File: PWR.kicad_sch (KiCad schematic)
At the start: 32 parts, among them J1 Conn_01x02_Pin, U2 XC6206P332MR, U4 MCP6001-OT, U5 AMS1117-3.3, U6 XL1509-5.0

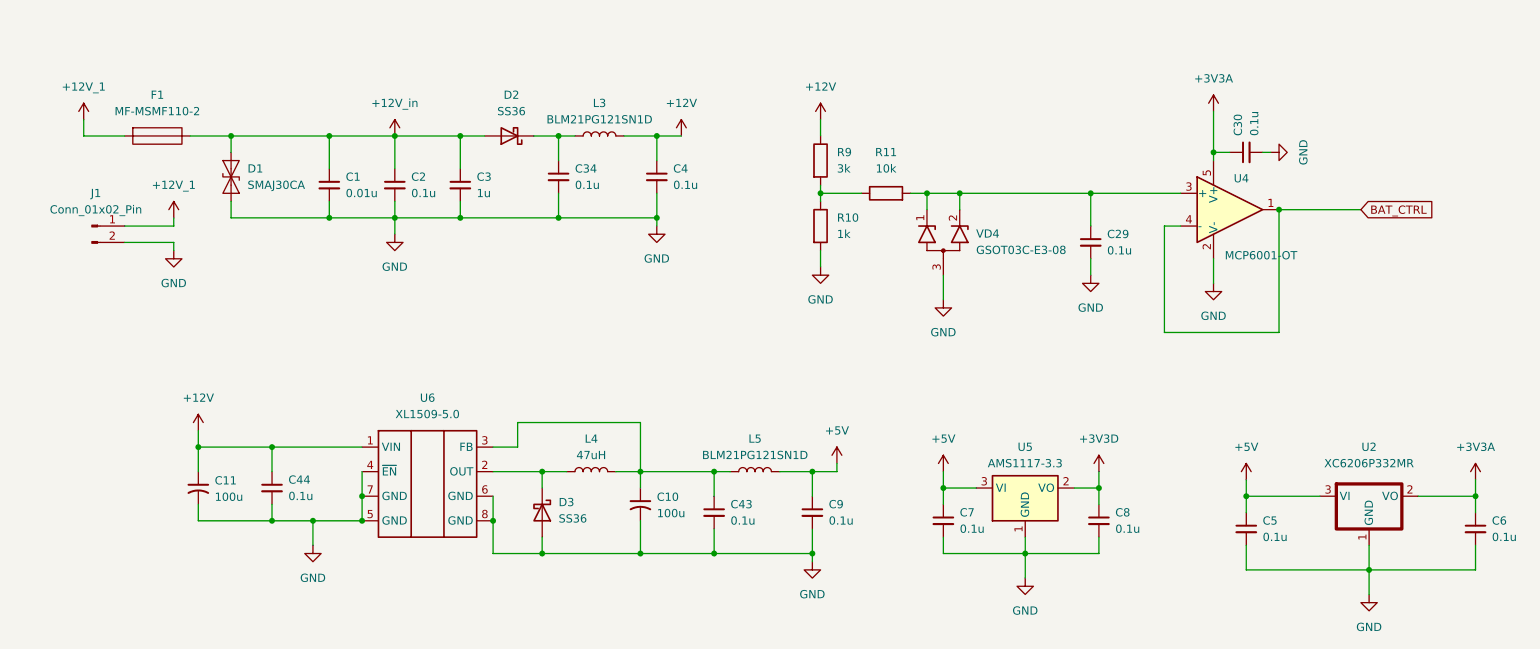
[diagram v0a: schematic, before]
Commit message: feat: начал работу над проектом пульта управления, продумана входная цепь питания устройства
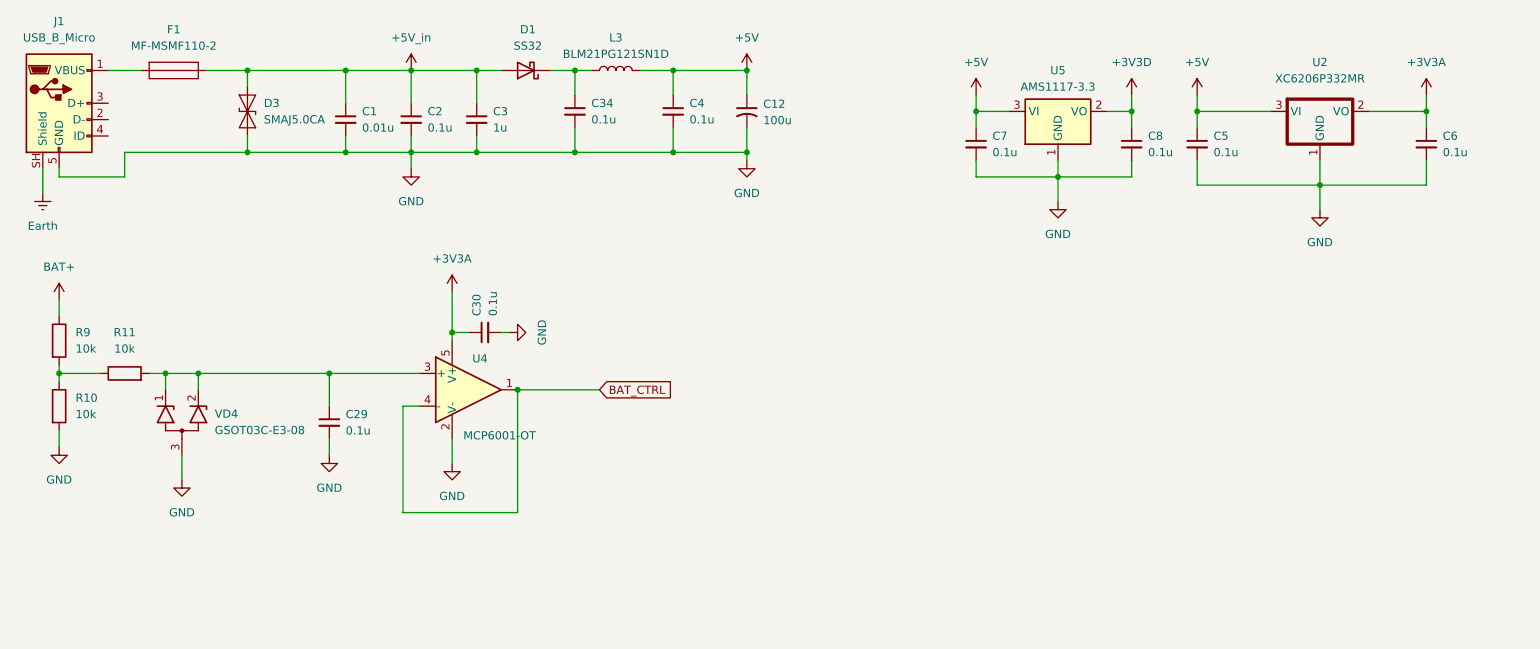
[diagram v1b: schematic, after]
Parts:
- removed C10, C11: 100u, Capacitor_SMD:C_Elec_6.3x7.7, symbol Device:C_Small_US
- removed C43, C44, C9: 0.1u, Capacitor_SMD:C_0805_2012Metric_Pad1.18x1.45mm_HandSolder, symbol Device:C_Small
- removed D1: SMAJ30CA, Diode_SMD:D_SMA, symbol Diode:SMAJ30CA
- removed D2, D3: SS36, Diode_SMD:D_SMA, symbol Diode:SS36
- removed J1: Conn_01x02_Pin, Connector_PinHeader_2.54mm:PinHeader_1x02_P2.54mm_Vertical, symbol Connector:Conn_01x02_Pin
- removed L4: 47uH, Inductor_SMD:L_12x12mm_H8mm, symbol Inductors:L
- removed L5: BLM21PG121SN1D, Inductor_SMD:L_0805_2012Metric_Pad1.05x1.20mm_HandSolder, symbol Inductors:L
- removed U6: XL1509-5.0, Package_SO:SOIC-8-1EP_3.9x4.9mm_P1.27mm_EP2.29x3mm_ThermalVias, symbol Power_suply:XL1509-5.0
- added C12: 100u, Capacitor_SMD:C_Elec_6.3x7.7, symbol Device:C_Small_US
- added D1: SS32, Diode_SMD:D_SMA, symbol Diode:SS32
- added D3: SMAJ5.0CA, Diode_SMD:D_SMA, symbol Diode:SMAJ5.0CA
- added J1: USB_B_Micro, Connector_USB:USB_Micro-B_Wuerth_629105150521, symbol Connector:USB_B_Micro
- R10: value 1k -> 10k
- R9: value 3k -> 10k
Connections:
- net +5V: now also C4.1, L3.2, C12.1
- net GND: now also C12.2, D3.1 (A1), J1.5 (GND)
- net at C34.1, L3.1: now also D1.1 (K)
- removed net +12V: C4.1, L3.2, R9.1
- net +12V_1: no longer names the net of F1.1 (A1)
- net +12V_1: now also J1.1 (VBUS)
- net +12V_in renamed +5V_in
- net +5V_in: now also D1.2 (A), D3.2 (A2)
- new net BAT+: R9.1
- new net Earth: J1.SH (Shield)
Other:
- moved on the sheet: C1, C2, C29, C3, C30, C34, C4, C5, C6, C7, C8, F1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
